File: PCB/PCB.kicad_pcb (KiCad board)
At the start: 2 copper layers, 182.9 x 104.1 mm, 33 parts, among them SW1 SW_Push, SW2 SW_Push, SW3 SW_Push, SW4 SW_Push, SW5 SW_Push, SW6 SW_Push, SW7 SW_Push, SW8 SW_Push

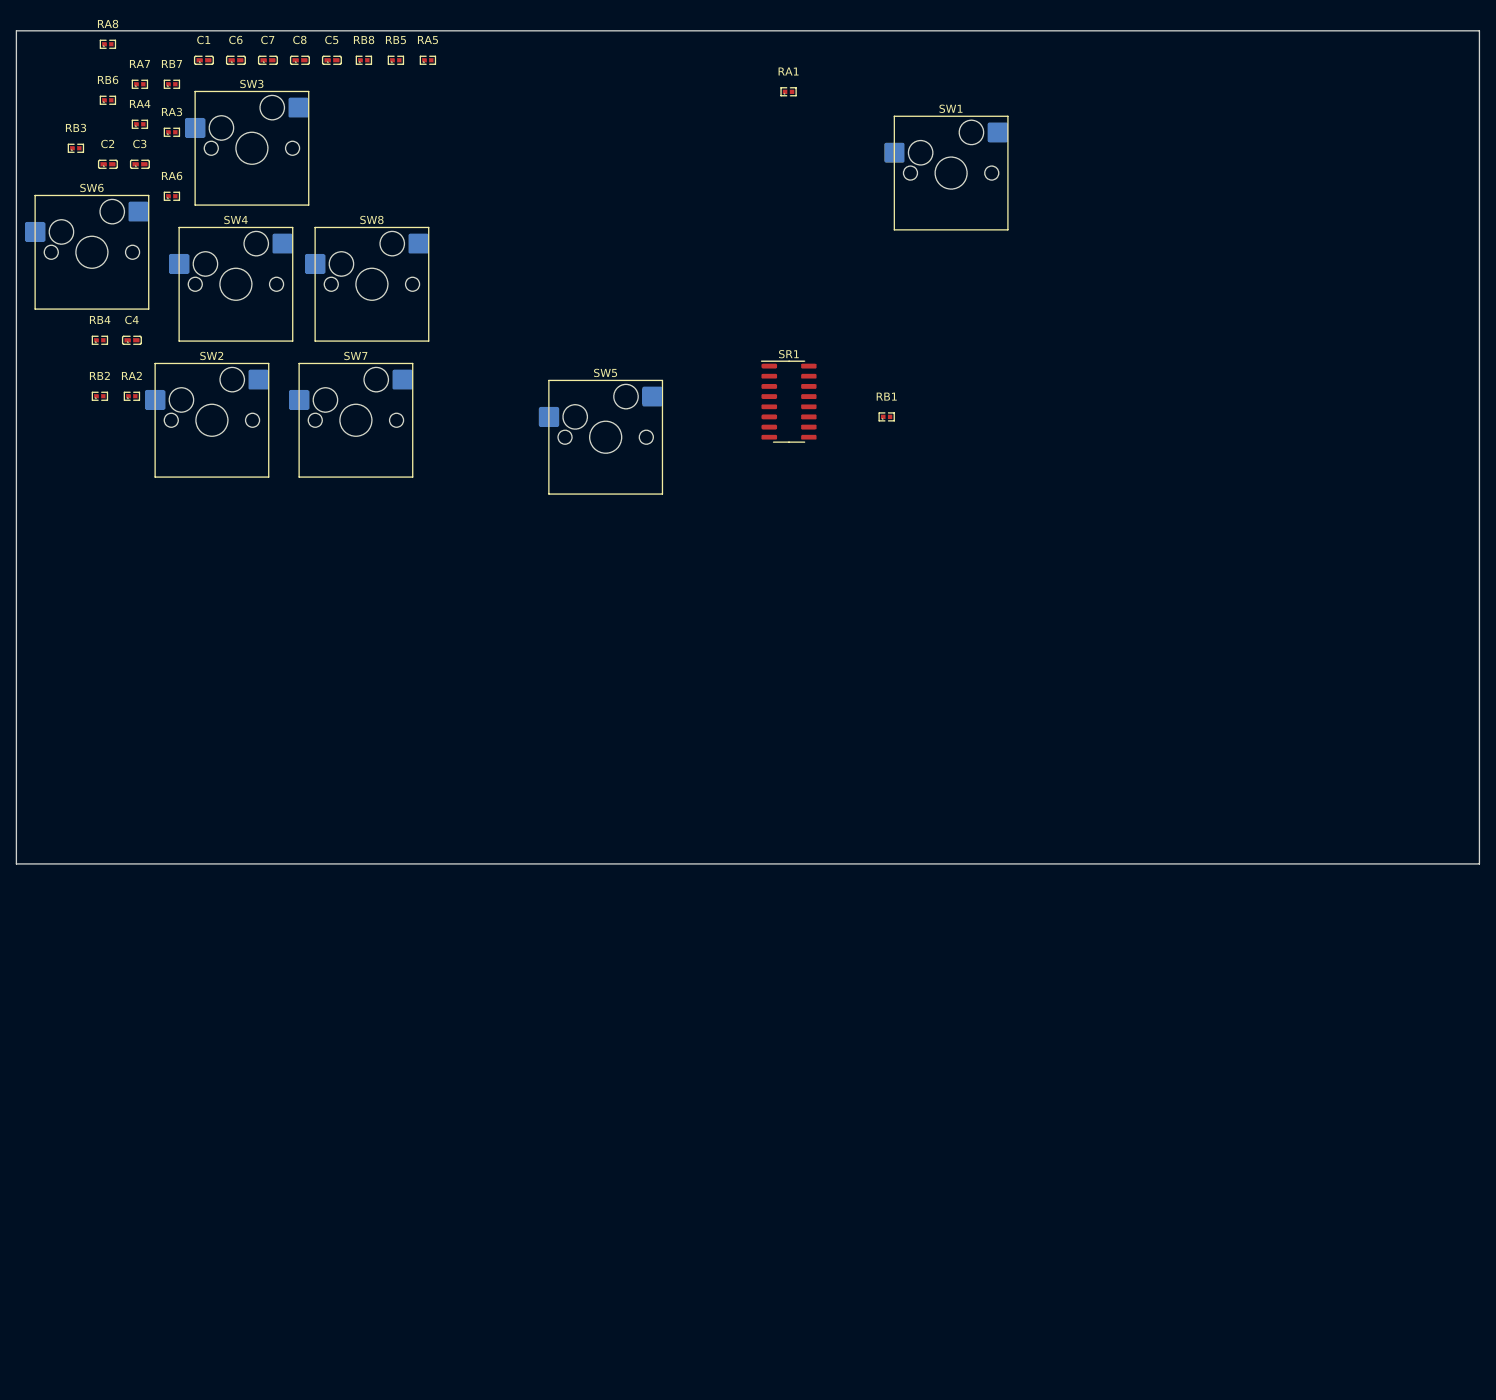
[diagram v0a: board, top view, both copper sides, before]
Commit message: Ready to work on PCB
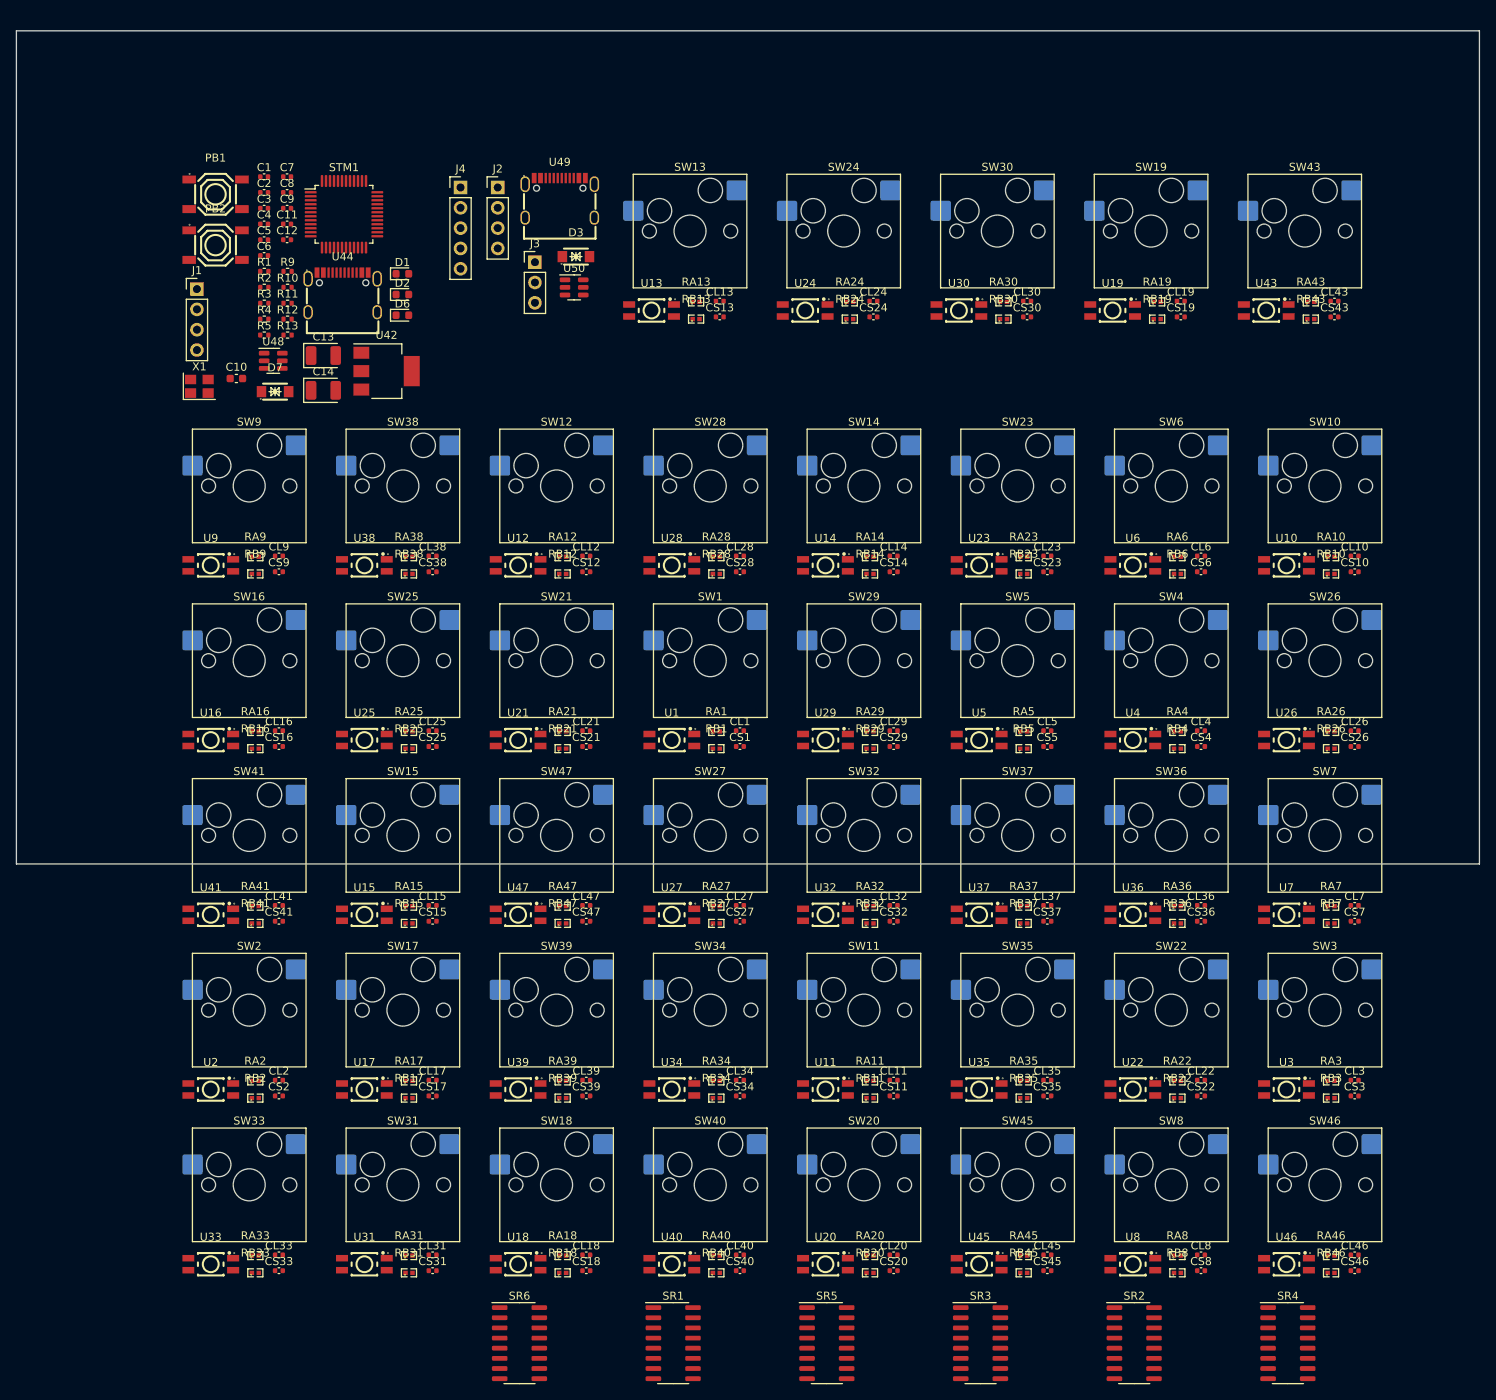
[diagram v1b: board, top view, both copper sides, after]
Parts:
- added C10: 4.7uF, Capacitor_SMD:C_0603_1608Metric, F.Cu at (63.1, 63.8)
- added C11: 100nF, Capacitor_SMD:C_0402_1005Metric, F.Cu at (69.4, 44.5)
- added C12: 100nF, Capacitor_SMD:C_0402_1005Metric, F.Cu at (69.4, 46.4)
- added C13: 100uF, Capacitor_Tantalum_SMD:CP_EIA-3528-15_AVX-H, F.Cu at (73.9, 60.9)
- added C14: 100uF, Capacitor_Tantalum_SMD:CP_EIA-3528-15_AVX-H, F.Cu at (73.9, 65.3)
- added C9: 1uF, Capacitor_SMD:C_0402_1005Metric, F.Cu at (69.4, 42.5)
- added CL1: 100nF, Capacitor_SMD:C_0402_1005Metric, F.Cu at (126.0, 107.8)
- added CL10: 100nF, Capacitor_SMD:C_0402_1005Metric, F.Cu at (202.8, 86.0)
- added CL11: 100nF, Capacitor_SMD:C_0402_1005Metric, F.Cu at (145.2, 151.5)
- added CL12: 100nF, Capacitor_SMD:C_0402_1005Metric, F.Cu at (106.8, 86.0)
- added CL13: 100nF, Capacitor_SMD:C_0402_1005Metric, F.Cu at (123.5, 54.1)
- added CL14: 100nF, Capacitor_SMD:C_0402_1005Metric, F.Cu at (145.2, 86.0)
- added CL15: 100nF, Capacitor_SMD:C_0402_1005Metric, F.Cu at (87.6, 129.7)
- added CL16: 100nF, Capacitor_SMD:C_0402_1005Metric, F.Cu at (68.4, 107.8)
- added CL17: 100nF, Capacitor_SMD:C_0402_1005Metric, F.Cu at (87.6, 151.5)
- added CL18: 100nF, Capacitor_SMD:C_0402_1005Metric, F.Cu at (106.8, 173.3)
- added CL19: 100nF, Capacitor_SMD:C_0402_1005Metric, F.Cu at (181.1, 54.1)
- added CL2: 100nF, Capacitor_SMD:C_0402_1005Metric, F.Cu at (68.4, 151.5)
- added CL20: 100nF, Capacitor_SMD:C_0402_1005Metric, F.Cu at (145.2, 173.3)
- added CL21: 100nF, Capacitor_SMD:C_0402_1005Metric, F.Cu at (106.8, 107.8)
- added CL22: 100nF, Capacitor_SMD:C_0402_1005Metric, F.Cu at (183.6, 151.5)
- added CL23: 100nF, Capacitor_SMD:C_0402_1005Metric, F.Cu at (164.4, 86.0)
- added CL24: 100nF, Capacitor_SMD:C_0402_1005Metric, F.Cu at (142.7, 54.1)
- added CL25: 100nF, Capacitor_SMD:C_0402_1005Metric, F.Cu at (87.6, 107.8)
- added CL26: 100nF, Capacitor_SMD:C_0402_1005Metric, F.Cu at (202.8, 107.8)
- added CL27: 100nF, Capacitor_SMD:C_0402_1005Metric, F.Cu at (126.0, 129.7)
- added CL28: 100nF, Capacitor_SMD:C_0402_1005Metric, F.Cu at (126.0, 86.0)
- added CL29: 100nF, Capacitor_SMD:C_0402_1005Metric, F.Cu at (145.2, 107.8)
- added CL3: 100nF, Capacitor_SMD:C_0402_1005Metric, F.Cu at (202.8, 151.5)
- added CL30: 100nF, Capacitor_SMD:C_0402_1005Metric, F.Cu at (161.9, 54.1)
- added CL31: 100nF, Capacitor_SMD:C_0402_1005Metric, F.Cu at (87.6, 173.3)
- added CL32: 100nF, Capacitor_SMD:C_0402_1005Metric, F.Cu at (145.2, 129.7)
- added CL33: 100nF, Capacitor_SMD:C_0402_1005Metric, F.Cu at (68.4, 173.3)
- added CL34: 100nF, Capacitor_SMD:C_0402_1005Metric, F.Cu at (126.0, 151.5)
- added CL35: 100nF, Capacitor_SMD:C_0402_1005Metric, F.Cu at (164.4, 151.5)
- added CL36: 100nF, Capacitor_SMD:C_0402_1005Metric, F.Cu at (183.6, 129.7)
- added CL37: 100nF, Capacitor_SMD:C_0402_1005Metric, F.Cu at (164.4, 129.7)
- added CL38: 100nF, Capacitor_SMD:C_0402_1005Metric, F.Cu at (87.6, 86.0)
- added CL39: 100nF, Capacitor_SMD:C_0402_1005Metric, F.Cu at (106.8, 151.5)
- added CL4: 100nF, Capacitor_SMD:C_0402_1005Metric, F.Cu at (183.6, 107.8)
- added CL40: 100nF, Capacitor_SMD:C_0402_1005Metric, F.Cu at (126.0, 173.3)
- added CL41: 100nF, Capacitor_SMD:C_0402_1005Metric, F.Cu at (68.4, 129.7)
- added CL43: 100nF, Capacitor_SMD:C_0402_1005Metric, F.Cu at (200.3, 54.1)
- added CL45: 100nF, Capacitor_SMD:C_0402_1005Metric, F.Cu at (164.4, 173.3)
- added CL46: 100nF, Capacitor_SMD:C_0402_1005Metric, F.Cu at (202.8, 173.3)
- added CL47: 100nF, Capacitor_SMD:C_0402_1005Metric, F.Cu at (106.8, 129.7)
- added CL5: 100nF, Capacitor_SMD:C_0402_1005Metric, F.Cu at (164.4, 107.8)
- added CL6: 100nF, Capacitor_SMD:C_0402_1005Metric, F.Cu at (183.6, 86.0)
- added CL7: 100nF, Capacitor_SMD:C_0402_1005Metric, F.Cu at (202.8, 129.7)
- added CL8: 100nF, Capacitor_SMD:C_0402_1005Metric, F.Cu at (183.6, 173.3)
- added CL9: 100nF, Capacitor_SMD:C_0402_1005Metric, F.Cu at (68.4, 86.0)
- added CS1: 100nF, Capacitor_SMD:C_0402_1005Metric, F.Cu at (126.0, 109.8)
- added CS10: 100nF, Capacitor_SMD:C_0402_1005Metric, F.Cu at (202.8, 87.9)
- added CS11: 100nF, Capacitor_SMD:C_0402_1005Metric, F.Cu at (145.2, 153.5)
- added CS12: 100nF, Capacitor_SMD:C_0402_1005Metric, F.Cu at (106.8, 87.9)
- added CS13: 100nF, Capacitor_SMD:C_0402_1005Metric, F.Cu at (123.5, 56.1)
- added CS14: 100nF, Capacitor_SMD:C_0402_1005Metric, F.Cu at (145.2, 87.9)
- added CS15: 100nF, Capacitor_SMD:C_0402_1005Metric, F.Cu at (87.6, 131.6)
- added CS16: 100nF, Capacitor_SMD:C_0402_1005Metric, F.Cu at (68.4, 109.8)
- added CS17: 100nF, Capacitor_SMD:C_0402_1005Metric, F.Cu at (87.6, 153.5)
- added CS18: 100nF, Capacitor_SMD:C_0402_1005Metric, F.Cu at (106.8, 175.3)
- added CS19: 100nF, Capacitor_SMD:C_0402_1005Metric, F.Cu at (181.1, 56.1)
- added CS2: 100nF, Capacitor_SMD:C_0402_1005Metric, F.Cu at (68.4, 153.5)
- added CS20: 100nF, Capacitor_SMD:C_0402_1005Metric, F.Cu at (145.2, 175.3)
- added CS21: 100nF, Capacitor_SMD:C_0402_1005Metric, F.Cu at (106.8, 109.8)
- added CS22: 100nF, Capacitor_SMD:C_0402_1005Metric, F.Cu at (183.6, 153.5)
- added CS23: 100nF, Capacitor_SMD:C_0402_1005Metric, F.Cu at (164.4, 87.9)
- added CS24: 100nF, Capacitor_SMD:C_0402_1005Metric, F.Cu at (142.7, 56.1)
- added CS25: 100nF, Capacitor_SMD:C_0402_1005Metric, F.Cu at (87.6, 109.8)
- added CS26: 100nF, Capacitor_SMD:C_0402_1005Metric, F.Cu at (202.8, 109.8)
- added CS27: 100nF, Capacitor_SMD:C_0402_1005Metric, F.Cu at (126.0, 131.6)
- added CS28: 100nF, Capacitor_SMD:C_0402_1005Metric, F.Cu at (126.0, 87.9)
- added CS29: 100nF, Capacitor_SMD:C_0402_1005Metric, F.Cu at (145.2, 109.8)
- added CS3: 100nF, Capacitor_SMD:C_0402_1005Metric, F.Cu at (202.8, 153.5)
- added CS30: 100nF, Capacitor_SMD:C_0402_1005Metric, F.Cu at (161.9, 56.1)
- added CS31: 100nF, Capacitor_SMD:C_0402_1005Metric, F.Cu at (87.6, 175.3)
- added CS32: 100nF, Capacitor_SMD:C_0402_1005Metric, F.Cu at (145.2, 131.6)
- added CS33: 100nF, Capacitor_SMD:C_0402_1005Metric, F.Cu at (68.4, 175.3)
- added CS34: 100nF, Capacitor_SMD:C_0402_1005Metric, F.Cu at (126.0, 153.5)
- added CS35: 100nF, Capacitor_SMD:C_0402_1005Metric, F.Cu at (164.4, 153.5)
- added CS36: 100nF, Capacitor_SMD:C_0402_1005Metric, F.Cu at (183.6, 131.6)
- added CS37: 100nF, Capacitor_SMD:C_0402_1005Metric, F.Cu at (164.4, 131.6)
- added CS38: 100nF, Capacitor_SMD:C_0402_1005Metric, F.Cu at (87.6, 87.9)
- added CS39: 100nF, Capacitor_SMD:C_0402_1005Metric, F.Cu at (106.8, 153.5)
- added CS4: 100nF, Capacitor_SMD:C_0402_1005Metric, F.Cu at (183.6, 109.8)
- added CS40: 100nF, Capacitor_SMD:C_0402_1005Metric, F.Cu at (126.0, 175.3)
- added CS41: 100nF, Capacitor_SMD:C_0402_1005Metric, F.Cu at (68.4, 131.6)
- added CS43: 100nF, Capacitor_SMD:C_0402_1005Metric, F.Cu at (200.3, 56.1)
- added CS45: 100nF, Capacitor_SMD:C_0402_1005Metric, F.Cu at (164.4, 175.3)
- added CS46: 100nF, Capacitor_SMD:C_0402_1005Metric, F.Cu at (202.8, 175.3)
- added CS47: 100nF, Capacitor_SMD:C_0402_1005Metric, F.Cu at (106.8, 131.6)
- added CS5: 100nF, Capacitor_SMD:C_0402_1005Metric, F.Cu at (164.4, 109.8)
- added CS6: 100nF, Capacitor_SMD:C_0402_1005Metric, F.Cu at (183.6, 87.9)
- added CS7: 100nF, Capacitor_SMD:C_0402_1005Metric, F.Cu at (202.8, 131.6)
- added CS8: 100nF, Capacitor_SMD:C_0402_1005Metric, F.Cu at (183.6, 175.3)
- added CS9: 100nF, Capacitor_SMD:C_0402_1005Metric, F.Cu at (68.4, 87.9)
- added D1: Red, LED_SMD:LED_0603_1608Metric, F.Cu at (83.8, 50.7)
- added D2: Red, LED_SMD:LED_0603_1608Metric, F.Cu at (83.8, 53.3)
- added D3: 6V ESD, footprint:SOD-123FL_L2.8-W1.8-LS3.7-BI, F.Cu at (105.5, 48.5)
- added D6: Red, LED_SMD:LED_0603_1608Metric, F.Cu at (83.8, 55.9)
- added D7: 6V ESD, footprint:SOD-123FL_L2.8-W1.8-LS3.7-BI, F.Cu at (67.9, 65.4)
- added J1: Debug, Connector_PinHeader_2.54mm:PinHeader_1x04_P2.54mm_Vertical, F.Cu at (58.1, 52.6)
- added J2: I2C, Connector_PinHeader_2.54mm:PinHeader_1x04_P2.54mm_Vertical, F.Cu at (95.7, 39.9)
- added J3: ALS, Connector_PinHeader_2.54mm:PinHeader_1x03_P2.54mm_Vertical, F.Cu at (100.4, 49.2)
- added J4: Serial, Connector_PinHeader_2.54mm:PinHeader_1x05_P2.54mm_Vertical, F.Cu at (91.1, 39.9)
- added PB1: TS-1187A-B-A-B, footprint:SW-SMD_4P-L5.1-W5.1-P3.70-LS6.5-TL-2, F.Cu at (60.5, 40.8)
- added PB2: TS-1187A-B-A-B, footprint:SW-SMD_4P-L5.1-W5.1-P3.70-LS6.5-TL-2, F.Cu at (60.5, 47.1)
- added R1: 15k, Resistor_SMD:R_0402_1005Metric, F.Cu at (66.5, 50.4)
- added R10: 5.1k, Resistor_SMD:R_0402_1005Metric, F.Cu at (69.5, 52.4)
- added R11: 5.1k, Resistor_SMD:R_0402_1005Metric, F.Cu at (69.5, 54.4)
- added R12: 5.1k, Resistor_SMD:R_0402_1005Metric, F.Cu at (69.5, 56.4)
- added R13: 1.5k, Resistor_SMD:R_0402_1005Metric, F.Cu at (69.5, 58.4)
- added R2: 15k, Resistor_SMD:R_0402_1005Metric, F.Cu at (66.5, 52.4)
- added R3: 15k, Resistor_SMD:R_0402_1005Metric, F.Cu at (66.5, 54.4)
- added R4: 5.1k, Resistor_SMD:R_0402_1005Metric, F.Cu at (66.5, 56.4)
- added R5: 1.5k, Resistor_SMD:R_0402_1005Metric, F.Cu at (66.5, 58.4)
- added R9: 5.1k, Resistor_SMD:R_0402_1005Metric, F.Cu at (69.5, 50.4)
- added RA10: 68kΩ, footprint:R0402, F.Cu at (199.9, 86.1)
- added RA11: 68kΩ, footprint:R0402, F.Cu at (142.3, 151.6)
- added RA12: 68kΩ, footprint:R0402, F.Cu at (103.8, 86.1)
- added RA13: 68kΩ, footprint:R0402, F.Cu at (120.5, 54.2)
- added RA14: 68kΩ, footprint:R0402, F.Cu at (142.3, 86.1)
- added RA15: 68kΩ, footprint:R0402, F.Cu at (84.6, 129.7)
- added RA16: 68kΩ, footprint:R0402, F.Cu at (65.4, 107.9)
- added RA17: 68kΩ, footprint:R0402, F.Cu at (84.6, 151.6)
- added RA18: 68kΩ, footprint:R0402, F.Cu at (103.8, 173.4)
- added RA19: 68kΩ, footprint:R0402, F.Cu at (178.2, 54.2)
- added RA20: 68kΩ, footprint:R0402, F.Cu at (142.3, 173.4)
- added RA21: 68kΩ, footprint:R0402, F.Cu at (103.8, 107.9)
- added RA22: 68kΩ, footprint:R0402, F.Cu at (180.7, 151.6)
- added RA23: 68kΩ, footprint:R0402, F.Cu at (161.5, 86.1)
- added RA24: 68kΩ, footprint:R0402, F.Cu at (139.7, 54.2)
- added RA25: 68kΩ, footprint:R0402, F.Cu at (84.6, 107.9)
- added RA26: 68kΩ, footprint:R0402, F.Cu at (199.9, 107.9)
- added RA27: 68kΩ, footprint:R0402, F.Cu at (123.1, 129.7)
- added RA28: 68kΩ, footprint:R0402, F.Cu at (123.1, 86.1)
- added RA29: 68kΩ, footprint:R0402, F.Cu at (142.3, 107.9)
- added RA30: 68kΩ, footprint:R0402, F.Cu at (158.9, 54.2)
- added RA31: 68kΩ, footprint:R0402, F.Cu at (84.6, 173.4)
- added RA32: 68kΩ, footprint:R0402, F.Cu at (142.3, 129.7)
- added RA33: 68kΩ, footprint:R0402, F.Cu at (65.4, 173.4)
- added RA34: 68kΩ, footprint:R0402, F.Cu at (123.1, 151.6)
- added RA35: 68kΩ, footprint:R0402, F.Cu at (161.5, 151.6)
- added RA36: 68kΩ, footprint:R0402, F.Cu at (180.7, 129.7)
- added RA37: 68kΩ, footprint:R0402, F.Cu at (161.5, 129.7)
- added RA38: 68kΩ, footprint:R0402, F.Cu at (84.6, 86.1)
- added RA39: 68kΩ, footprint:R0402, F.Cu at (103.8, 151.6)
- added RA40: 68kΩ, footprint:R0402, F.Cu at (123.1, 173.4)
- added RA41: 68kΩ, footprint:R0402, F.Cu at (65.4, 129.7)
- added RA43: 68kΩ, footprint:R0402, F.Cu at (197.4, 54.2)
- added RA45: 68kΩ, footprint:R0402, F.Cu at (161.5, 173.4)
- added RA46: 68kΩ, footprint:R0402, F.Cu at (199.9, 173.4)
- added RA47: 68kΩ, footprint:R0402, F.Cu at (103.8, 129.7)
- added RA9: 68kΩ, footprint:R0402, F.Cu at (65.4, 86.1)
- added RB10: 33kΩ, footprint:R0402, F.Cu at (199.9, 88.2)
- added RB11: 33kΩ, footprint:R0402, F.Cu at (142.3, 153.7)
- added RB12: 33kΩ, footprint:R0402, F.Cu at (103.8, 88.2)
- added RB13: 33kΩ, footprint:R0402, F.Cu at (120.5, 56.3)
- added RB14: 33kΩ, footprint:R0402, F.Cu at (142.3, 88.2)
- added RB15: 33kΩ, footprint:R0402, F.Cu at (84.6, 131.9)
- added RB16: 33kΩ, footprint:R0402, F.Cu at (65.4, 110.0)
- added RB17: 33kΩ, footprint:R0402, F.Cu at (84.6, 153.7)
- added RB18: 33kΩ, footprint:R0402, F.Cu at (103.8, 175.6)
- added RB19: 33kΩ, footprint:R0402, F.Cu at (178.2, 56.3)
- added RB20: 33kΩ, footprint:R0402, F.Cu at (142.3, 175.6)
- added RB21: 33kΩ, footprint:R0402, F.Cu at (103.8, 110.0)
- added RB22: 33kΩ, footprint:R0402, F.Cu at (180.7, 153.7)
- added RB23: 33kΩ, footprint:R0402, F.Cu at (161.5, 88.2)
- added RB24: 33kΩ, footprint:R0402, F.Cu at (139.7, 56.3)
- added RB25: 33kΩ, footprint:R0402, F.Cu at (84.6, 110.0)
- added RB26: 33kΩ, footprint:R0402, F.Cu at (199.9, 110.0)
- added RB27: 33kΩ, footprint:R0402, F.Cu at (123.1, 131.9)
- added RB28: 33kΩ, footprint:R0402, F.Cu at (123.1, 88.2)
- added RB29: 33kΩ, footprint:R0402, F.Cu at (142.3, 110.0)
- added RB30: 33kΩ, footprint:R0402, F.Cu at (158.9, 56.3)
- added RB31: 33kΩ, footprint:R0402, F.Cu at (84.6, 175.6)
- added RB32: 33kΩ, footprint:R0402, F.Cu at (142.3, 131.9)
- added RB33: 33kΩ, footprint:R0402, F.Cu at (65.4, 175.6)
- added RB34: 33kΩ, footprint:R0402, F.Cu at (123.1, 153.7)
- added RB35: 33kΩ, footprint:R0402, F.Cu at (161.5, 153.7)
- added RB36: 33kΩ, footprint:R0402, F.Cu at (180.7, 131.9)
- added RB37: 33kΩ, footprint:R0402, F.Cu at (161.5, 131.9)
- added RB38: 33kΩ, footprint:R0402, F.Cu at (84.6, 88.2)
- added RB39: 33kΩ, footprint:R0402, F.Cu at (103.8, 153.7)
- added RB40: 33kΩ, footprint:R0402, F.Cu at (123.1, 175.6)
- added RB41: 33kΩ, footprint:R0402, F.Cu at (65.4, 131.9)
- added RB43: 33kΩ, footprint:R0402, F.Cu at (197.4, 56.3)
- added RB45: 33kΩ, footprint:R0402, F.Cu at (161.5, 175.6)
- added RB46: 33kΩ, footprint:R0402, F.Cu at (199.9, 175.6)
- added RB47: 33kΩ, footprint:R0402, F.Cu at (103.8, 131.9)
- added RB9: 33kΩ, footprint:R0402, F.Cu at (65.4, 88.2)
- added SR2: 74HC165, Package_SO:SOIC-16_3.9x9.9mm_P1.27mm, F.Cu at (175.3, 184.4)
- added SR3: 74HC165, Package_SO:SOIC-16_3.9x9.9mm_P1.27mm, F.Cu at (156.1, 184.4)
- added SR4: 74HC165, Package_SO:SOIC-16_3.9x9.9mm_P1.27mm, F.Cu at (194.5, 184.4)
- added SR5: 74HC165, Package_SO:SOIC-16_3.9x9.9mm_P1.27mm, F.Cu at (136.9, 184.4)
- added SR6: 74HC165, Package_SO:SOIC-16_3.9x9.9mm_P1.27mm, F.Cu at (98.4, 184.4)
- added STM1: STM32F103C8Tx, Package_QFP:LQFP-48_7x7mm_P0.5mm, F.Cu at (76.5, 43.2)
- added SW10: SW_Push, PCM_Switch_Keyboard_Hotswap_Kailh:SW_Hotswap_Kailh_MX, F.Cu at (199.1, 77.2)
- added SW11: SW_Push, PCM_Switch_Keyboard_Hotswap_Kailh:SW_Hotswap_Kailh_MX, F.Cu at (141.5, 142.7)
- added SW12: SW_Push, PCM_Switch_Keyboard_Hotswap_Kailh:SW_Hotswap_Kailh_MX, F.Cu at (103.1, 77.2)
- added SW13: SW_Push, PCM_Switch_Keyboard_Hotswap_Kailh:SW_Hotswap_Kailh_MX, F.Cu at (119.8, 45.4)
- added SW14: SW_Push, PCM_Switch_Keyboard_Hotswap_Kailh:SW_Hotswap_Kailh_MX, F.Cu at (141.5, 77.2)
- added SW15: SW_Push, PCM_Switch_Keyboard_Hotswap_Kailh:SW_Hotswap_Kailh_MX, F.Cu at (83.9, 120.9)
- added SW16: SW_Push, PCM_Switch_Keyboard_Hotswap_Kailh:SW_Hotswap_Kailh_MX, F.Cu at (64.7, 99.0)
- added SW17: SW_Push, PCM_Switch_Keyboard_Hotswap_Kailh:SW_Hotswap_Kailh_MX, F.Cu at (83.9, 142.7)
- added SW18: SW_Push, PCM_Switch_Keyboard_Hotswap_Kailh:SW_Hotswap_Kailh_MX, F.Cu at (103.1, 164.6)
- added SW19: SW_Push, PCM_Switch_Keyboard_Hotswap_Kailh:SW_Hotswap_Kailh_MX, F.Cu at (177.4, 45.4)
- added SW20: SW_Push, PCM_Switch_Keyboard_Hotswap_Kailh:SW_Hotswap_Kailh_MX, F.Cu at (141.5, 164.6)
- added SW21: SW_Push, PCM_Switch_Keyboard_Hotswap_Kailh:SW_Hotswap_Kailh_MX, F.Cu at (103.1, 99.0)
- added SW22: SW_Push, PCM_Switch_Keyboard_Hotswap_Kailh:SW_Hotswap_Kailh_MX, F.Cu at (179.9, 142.7)
- added SW23: SW_Push, PCM_Switch_Keyboard_Hotswap_Kailh:SW_Hotswap_Kailh_MX, F.Cu at (160.7, 77.2)
- added SW24: SW_Push, PCM_Switch_Keyboard_Hotswap_Kailh:SW_Hotswap_Kailh_MX, F.Cu at (139.0, 45.4)
- added SW25: SW_Push, PCM_Switch_Keyboard_Hotswap_Kailh:SW_Hotswap_Kailh_MX, F.Cu at (83.9, 99.0)
- added SW26: SW_Push, PCM_Switch_Keyboard_Hotswap_Kailh:SW_Hotswap_Kailh_MX, F.Cu at (199.1, 99.0)
- added SW27: SW_Push, PCM_Switch_Keyboard_Hotswap_Kailh:SW_Hotswap_Kailh_MX, F.Cu at (122.3, 120.9)
- added SW28: SW_Push, PCM_Switch_Keyboard_Hotswap_Kailh:SW_Hotswap_Kailh_MX, F.Cu at (122.3, 77.2)
- added SW29: SW_Push, PCM_Switch_Keyboard_Hotswap_Kailh:SW_Hotswap_Kailh_MX, F.Cu at (141.5, 99.0)
- added SW30: SW_Push, PCM_Switch_Keyboard_Hotswap_Kailh:SW_Hotswap_Kailh_MX, F.Cu at (158.2, 45.4)
- added SW31: SW_Push, PCM_Switch_Keyboard_Hotswap_Kailh:SW_Hotswap_Kailh_MX, F.Cu at (83.9, 164.6)
- added SW32: SW_Push, PCM_Switch_Keyboard_Hotswap_Kailh:SW_Hotswap_Kailh_MX, F.Cu at (141.5, 120.9)
- added SW33: SW_Push, PCM_Switch_Keyboard_Hotswap_Kailh:SW_Hotswap_Kailh_MX, F.Cu at (64.7, 164.6)
- added SW34: SW_Push, PCM_Switch_Keyboard_Hotswap_Kailh:SW_Hotswap_Kailh_MX, F.Cu at (122.3, 142.7)
- added SW35: SW_Push, PCM_Switch_Keyboard_Hotswap_Kailh:SW_Hotswap_Kailh_MX, F.Cu at (160.7, 142.7)
- added SW36: SW_Push, PCM_Switch_Keyboard_Hotswap_Kailh:SW_Hotswap_Kailh_MX, F.Cu at (179.9, 120.9)
- added SW37: SW_Push, PCM_Switch_Keyboard_Hotswap_Kailh:SW_Hotswap_Kailh_MX, F.Cu at (160.7, 120.9)
- added SW38: SW_Push, PCM_Switch_Keyboard_Hotswap_Kailh:SW_Hotswap_Kailh_MX, F.Cu at (83.9, 77.2)
- added SW39: SW_Push, PCM_Switch_Keyboard_Hotswap_Kailh:SW_Hotswap_Kailh_MX, F.Cu at (103.1, 142.7)
- added SW40: SW_Push, PCM_Switch_Keyboard_Hotswap_Kailh:SW_Hotswap_Kailh_MX, F.Cu at (122.3, 164.6)
- added SW41: SW_Push, PCM_Switch_Keyboard_Hotswap_Kailh:SW_Hotswap_Kailh_MX, F.Cu at (64.7, 120.9)
- added SW43: SW_Push, PCM_Switch_Keyboard_Hotswap_Kailh:SW_Hotswap_Kailh_MX, F.Cu at (196.6, 45.4)
- added SW45: SW_Push, PCM_Switch_Keyboard_Hotswap_Kailh:SW_Hotswap_Kailh_MX, F.Cu at (160.7, 164.6)
- added SW46: SW_Push, PCM_Switch_Keyboard_Hotswap_Kailh:SW_Hotswap_Kailh_MX, F.Cu at (199.1, 164.6)
- added SW47: SW_Push, PCM_Switch_Keyboard_Hotswap_Kailh:SW_Hotswap_Kailh_MX, F.Cu at (103.1, 120.9)
- added SW9: SW_Push, PCM_Switch_Keyboard_Hotswap_Kailh:SW_Hotswap_Kailh_MX, F.Cu at (64.7, 77.2)
- added U1: SK6812MINI-E_C5149201, footprint:LED-SMD_L3.2-W2.8-TR, F.Cu at (117.5, 109.0)
- added U10: SK6812MINI-E_C5149201, footprint:LED-SMD_L3.2-W2.8-TR, F.Cu at (194.3, 87.1)
- added U11: SK6812MINI-E_C5149201, footprint:LED-SMD_L3.2-W2.8-TR, F.Cu at (136.7, 152.7)
- added U12: SK6812MINI-E_C5149201, footprint:LED-SMD_L3.2-W2.8-TR, F.Cu at (98.3, 87.1)
- added U13: SK6812MINI-E_C5149201, footprint:LED-SMD_L3.2-W2.8-TR, F.Cu at (115.0, 55.3)
- added U14: SK6812MINI-E_C5149201, footprint:LED-SMD_L3.2-W2.8-TR, F.Cu at (136.7, 87.1)
- added U15: SK6812MINI-E_C5149201, footprint:LED-SMD_L3.2-W2.8-TR, F.Cu at (79.1, 130.8)
- added U16: SK6812MINI-E_C5149201, footprint:LED-SMD_L3.2-W2.8-TR, F.Cu at (59.9, 109.0)
- added U17: SK6812MINI-E_C5149201, footprint:LED-SMD_L3.2-W2.8-TR, F.Cu at (79.1, 152.7)
- added U18: SK6812MINI-E_C5149201, footprint:LED-SMD_L3.2-W2.8-TR, F.Cu at (98.3, 174.5)
- added U19: SK6812MINI-E_C5149201, footprint:LED-SMD_L3.2-W2.8-TR, F.Cu at (172.6, 55.3)
- added U2: SK6812MINI-E_C5149201, footprint:LED-SMD_L3.2-W2.8-TR, F.Cu at (59.9, 152.7)
- added U20: SK6812MINI-E_C5149201, footprint:LED-SMD_L3.2-W2.8-TR, F.Cu at (136.7, 174.5)
- added U21: SK6812MINI-E_C5149201, footprint:LED-SMD_L3.2-W2.8-TR, F.Cu at (98.3, 109.0)
- added U22: SK6812MINI-E_C5149201, footprint:LED-SMD_L3.2-W2.8-TR, F.Cu at (175.1, 152.7)
- added U23: SK6812MINI-E_C5149201, footprint:LED-SMD_L3.2-W2.8-TR, F.Cu at (155.9, 87.1)
- added U24: SK6812MINI-E_C5149201, footprint:LED-SMD_L3.2-W2.8-TR, F.Cu at (134.2, 55.3)
- added U25: SK6812MINI-E_C5149201, footprint:LED-SMD_L3.2-W2.8-TR, F.Cu at (79.1, 109.0)
- added U26: SK6812MINI-E_C5149201, footprint:LED-SMD_L3.2-W2.8-TR, F.Cu at (194.3, 109.0)
- added U27: SK6812MINI-E_C5149201, footprint:LED-SMD_L3.2-W2.8-TR, F.Cu at (117.5, 130.8)
- added U28: SK6812MINI-E_C5149201, footprint:LED-SMD_L3.2-W2.8-TR, F.Cu at (117.5, 87.1)
- added U29: SK6812MINI-E_C5149201, footprint:LED-SMD_L3.2-W2.8-TR, F.Cu at (136.7, 109.0)
- added U3: SK6812MINI-E_C5149201, footprint:LED-SMD_L3.2-W2.8-TR, F.Cu at (194.3, 152.7)
- added U30: SK6812MINI-E_C5149201, footprint:LED-SMD_L3.2-W2.8-TR, F.Cu at (153.4, 55.3)
- added U31: SK6812MINI-E_C5149201, footprint:LED-SMD_L3.2-W2.8-TR, F.Cu at (79.1, 174.5)
- added U32: SK6812MINI-E_C5149201, footprint:LED-SMD_L3.2-W2.8-TR, F.Cu at (136.7, 130.8)
- added U33: SK6812MINI-E_C5149201, footprint:LED-SMD_L3.2-W2.8-TR, F.Cu at (59.9, 174.5)
- added U34: SK6812MINI-E_C5149201, footprint:LED-SMD_L3.2-W2.8-TR, F.Cu at (117.5, 152.7)
- added U35: SK6812MINI-E_C5149201, footprint:LED-SMD_L3.2-W2.8-TR, F.Cu at (155.9, 152.7)
- added U36: SK6812MINI-E_C5149201, footprint:LED-SMD_L3.2-W2.8-TR, F.Cu at (175.1, 130.8)
- added U37: SK6812MINI-E_C5149201, footprint:LED-SMD_L3.2-W2.8-TR, F.Cu at (155.9, 130.8)
- added U38: SK6812MINI-E_C5149201, footprint:LED-SMD_L3.2-W2.8-TR, F.Cu at (79.1, 87.1)
- added U39: SK6812MINI-E_C5149201, footprint:LED-SMD_L3.2-W2.8-TR, F.Cu at (98.3, 152.7)
- added U4: SK6812MINI-E_C5149201, footprint:LED-SMD_L3.2-W2.8-TR, F.Cu at (175.1, 109.0)
- added U40: SK6812MINI-E_C5149201, footprint:LED-SMD_L3.2-W2.8-TR, F.Cu at (117.5, 174.5)
- added U41: SK6812MINI-E_C5149201, footprint:LED-SMD_L3.2-W2.8-TR, F.Cu at (59.9, 130.8)
- added U42: AMS1117-3.3, Package_TO_SOT_SMD:SOT-223-3_TabPin2, F.Cu at (81.8, 62.9)
- added U43: SK6812MINI-E_C5149201, footprint:LED-SMD_L3.2-W2.8-TR, F.Cu at (191.8, 55.3)
- added U44: TYPE-C-31-M-12, footprint:USB-C_SMD-TYPE-C-31-M-12, F.Cu at (76.3, 53.0)
- added U45: SK6812MINI-E_C5149201, footprint:LED-SMD_L3.2-W2.8-TR, F.Cu at (155.9, 174.5)
- added U46: SK6812MINI-E_C5149201, footprint:LED-SMD_L3.2-W2.8-TR, F.Cu at (194.3, 174.5)
- added U47: SK6812MINI-E_C5149201, footprint:LED-SMD_L3.2-W2.8-TR, F.Cu at (98.3, 130.8)
- added U48: USBLC6-2SC6, Package_TO_SOT_SMD:SOT-23-6, F.Cu at (67.7, 61.6)
- added U49: TYPE-C-31-M-12, footprint:USB-C_SMD-TYPE-C-31-M-12, F.Cu at (103.5, 41.2)
- added U5: SK6812MINI-E_C5149201, footprint:LED-SMD_L3.2-W2.8-TR, F.Cu at (155.9, 109.0)
- added U50: USBLC6-2SC6, Package_TO_SOT_SMD:SOT-23-6, F.Cu at (105.3, 52.4)
- added U6: SK6812MINI-E_C5149201, footprint:LED-SMD_L3.2-W2.8-TR, F.Cu at (175.1, 87.1)
- added U7: SK6812MINI-E_C5149201, footprint:LED-SMD_L3.2-W2.8-TR, F.Cu at (194.3, 130.8)
- added U8: SK6812MINI-E_C5149201, footprint:LED-SMD_L3.2-W2.8-TR, F.Cu at (175.1, 174.5)
- added U9: SK6812MINI-E_C5149201, footprint:LED-SMD_L3.2-W2.8-TR, F.Cu at (59.9, 87.1)
- added X1: Crystal, Crystal:Crystal_SMD_3225-4Pin_3.2x2.5mm, F.Cu at (58.4, 64.8)
- C1, C2: value 100nF -> 30pF; footprint footprint:C0402 -> Capacitor_SMD:C_0402_1005Metric
- C3, C4, C5, C6, C8: footprint footprint:C0402 -> Capacitor_SMD:C_0402_1005Metric
- C7: value 100nF -> 10nF; footprint footprint:C0402 -> Capacitor_SMD:C_0402_1005Metric
- moved RA8 202.0 mm to (180.7, 173.4)
- moved RB3 196.8 mm to (199.9, 153.7)
- moved RA3 187.2 mm to (199.9, 151.6)
- moved RB8 182.5 mm to (180.7, 175.6)
- moved RA7 180.9 mm to (199.9, 129.7)
- moved RB7 178.9 mm to (199.9, 131.9)
- moved SW3 172.0 mm to (199.1, 142.7)
- moved SW8 150.5 mm to (179.9, 164.6)
- moved RA4 150.3 mm to (180.7, 107.9)
- moved RB6 146.2 mm to (180.7, 88.2)
- moved RB4 144.0 mm to (180.7, 110.0)
- moved SW6 138.0 mm to (179.9, 77.2)
- moved RA6 133.5 mm to (180.7, 86.1)
- moved SW7 131.8 mm to (199.1, 120.9)
- moved SW4 126.0 mm to (179.9, 99.0)
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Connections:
- C1 pad 2: /Key Column/SW1 -> Net-(STM1-PD0)
- C2 pad 2: /Key Column/SW2 -> Net-(STM1-PD1)
- C3 pad 2: /Key Column/SW3 -> +3.3V
- C4 pad 2: /Key Column/SW4 -> +3.3V
- C5 pad 2: /Key Column/SW5 -> +3.3V
- C6 pad 2: /Key Column/SW6 -> +3.3V
- C7 pad 2: /Key Column/SW7 -> +3.3V
- C8 pad 2: /Key Column/SW8 -> +3.3V
- RB1 pad 1: /Key Column/SW1 -> /Left Half/8-Key Module1/Key Unit7/SwitchOutput
- RB2 pad 1: /Key Column/SW2 -> /Left Half/8-Key Module4/Key Unit3/SwitchOutput
- RB3 pad 1: /Key Column/SW3 -> /Left Half/8-Key Module/Key Unit2/SwitchOutput
- RB4 pad 1: /Key Column/SW4 -> /Left Half/8-Key Module2/Key Unit6/SwitchOutput
- RB5 pad 1: /Key Column/SW5 -> /Left Half/8-Key Module2/Key Unit0/SwitchOutput
- RB6 pad 1: /Key Column/SW6 -> /Left Half/8-Key Module1/Key Unit0/SwitchOutput
- RB7 pad 1: /Key Column/SW7 -> /Left Half/5-Key Module/Key Unit8/SwitchOutput
- RB8 pad 1: /Key Column/SW8 -> /Left Half/8-Key Module/Key Unit1/SwitchOutput
- SR1 pad 1: unconnected-(SR1-~{PL}-Pad1) -> /Left Half/5-Key Module/SR_LOAD
- SR1 pad 10: unconnected-(SR1-DS-Pad10) -> /Left Half/8-Key Module1/SR_OUT
- SR1 pad 11: /Key Column/SW1 -> /Left Half/8-Key Module2/Key Unit7/SwitchOutput
- SR1 pad 12: /Key Column/SW2 -> /Left Half/8-Key Module2/Key Unit6/SwitchOutput
- SR1 pad 13: /Key Column/SW3 -> /Left Half/8-Key Module2/Key Unit5/SwitchOutput
- SR1 pad 14: /Key Column/SW4 -> /Left Half/8-Key Module2/Key Unit4/SwitchOutput
- SR1 pad 2: unconnected-(SR1-CP-Pad2) -> /Left Half/5-Key Module/SR_CLOCK
- SR1 pad 3: /Key Column/SW5 -> /Left Half/8-Key Module2/Key Unit3/SwitchOutput
- SR1 pad 4: /Key Column/SW6 -> /Left Half/8-Key Module2/Key Unit2/SwitchOutput
- SR1 pad 5: /Key Column/SW7 -> /Left Half/8-Key Module2/Key Unit1/SwitchOutput
- SR1 pad 6: /Key Column/SW8 -> /Left Half/8-Key Module2/Key Unit0/SwitchOutput
- SR1 pad 9: unconnected-(SR1-Q7-Pad9) -> /Left Half/8-Key Module2/SR_OUT
